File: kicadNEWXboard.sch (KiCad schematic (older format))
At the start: 24 parts, among them SW1 SW_Push, U1 ATmega32U4-AU, Y1 16MHz

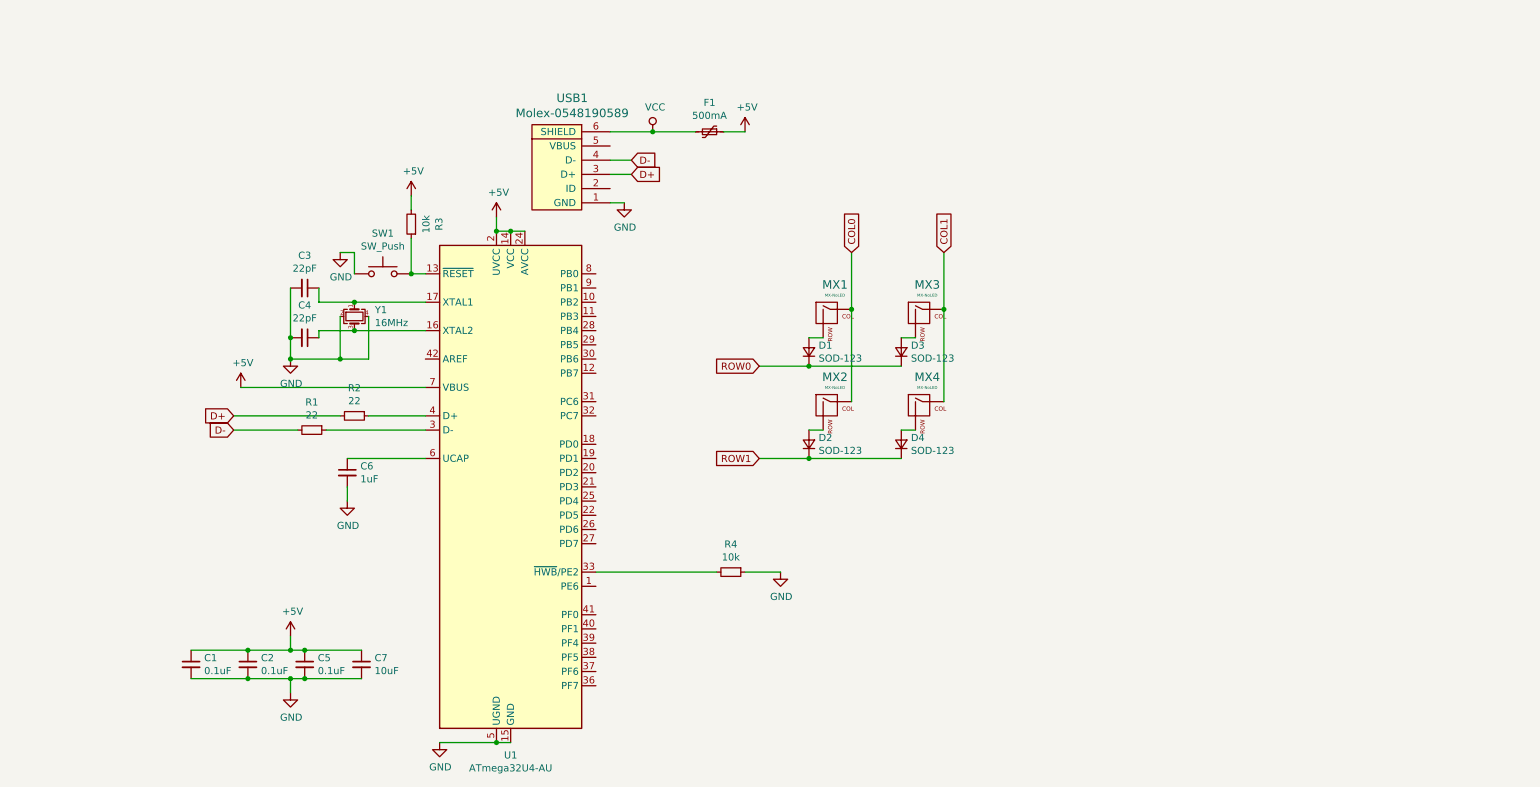
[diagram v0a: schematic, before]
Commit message: SVG
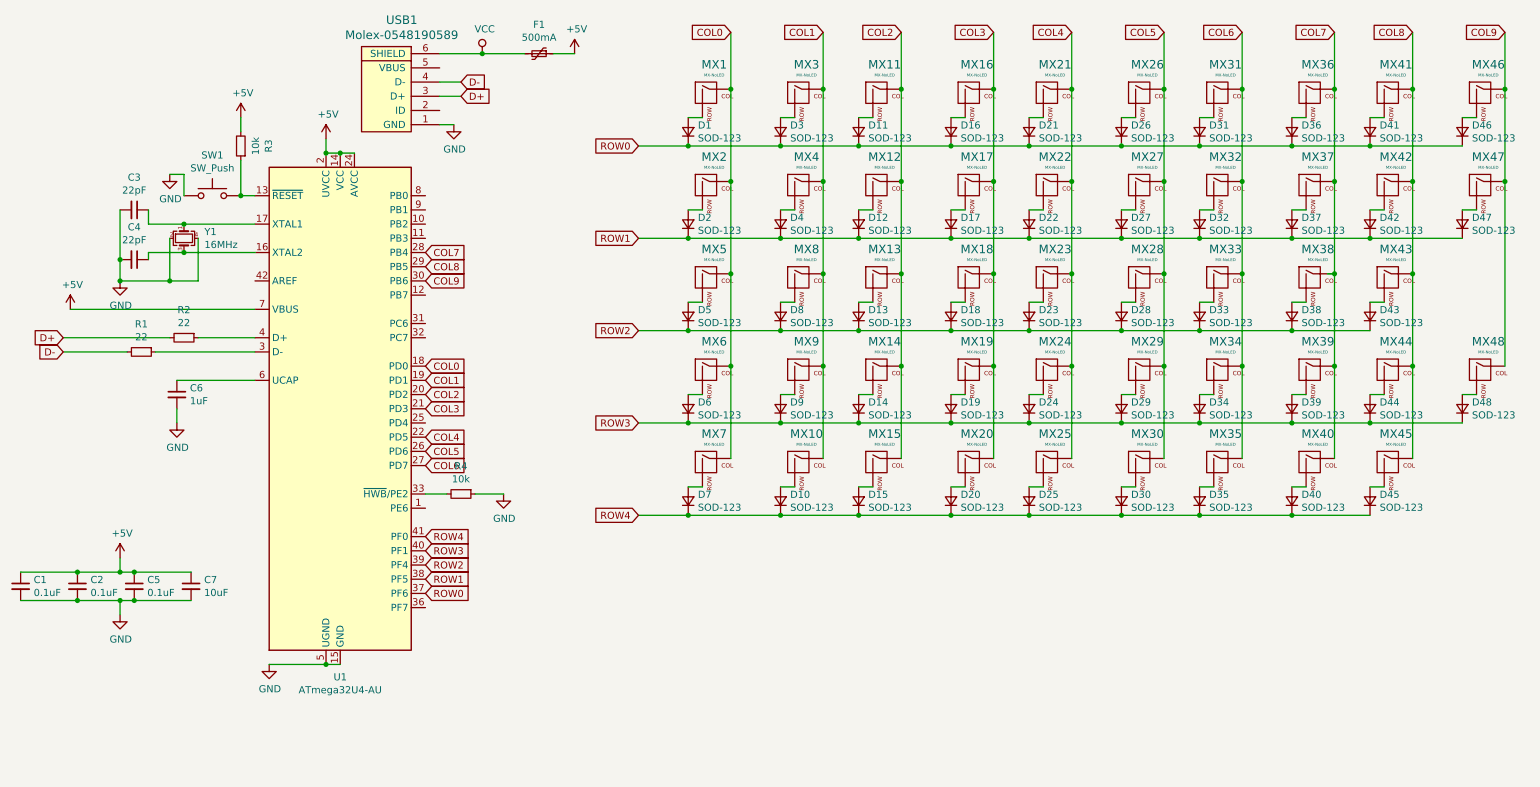
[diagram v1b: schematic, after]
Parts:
- added D10, D11, D12, D13, D14, D15, D16, D17, D18, D19, D20, D21, D22, D23, D24, D25, D26, D27, D28, D29, D30, D31, D32, D33, D34, D35, D36, D37, D38, D39, D40, D41, D42, D43, D44, D45, D46, D47, D48, D5, D6, D7, D8, D9: SOD-123, Diode_SMD:D_SOD-123, symbol Device:D_Small
- added MX10, MX11, MX12, MX13, MX14, MX15, MX16, MX17, MX18, MX19, MX20, MX21, MX22, MX23, MX24, MX25, MX26, MX27, MX28, MX29, MX30, MX31, MX32, MX33, MX34, MX35, MX36, MX37, MX38, MX39, MX40, MX41, MX42, MX43, MX44, MX45, MX46, MX47, MX48, MX5, MX6, MX7, MX8, MX9: MX-NoLED, MX_Alps_Hybrid:MX-1U, symbol MX_Alps_Hybrid:MX-NoLED
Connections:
- net COL0: now also U1.18 (PD0), MX5.1 (COL), MX6.1 (COL), MX7.1 (COL)
- net COL1: now also U1.19 (PD1), MX10.1 (COL), MX8.1 (COL), MX9.1 (COL)
- net ROW0: now also U1.37 (PF6), D11.1 (K), D16.1 (K), D21.1 (K), D26.1 (K), D31.1 (K), D36.1 (K), D41.1 (K), D46.1 (K)
- net ROW1: now also U1.38 (PF5), D12.1 (K), D17.1 (K), D22.1 (K), D27.1 (K), D32.1 (K), D37.1 (K), D42.1 (K), D47.1 (K)
- net COL2: now reaches U1.20 (PD2)
- net COL2: now also MX11.1 (COL), MX12.1 (COL), MX13.1 (COL), MX14.1 (COL), MX15.1 (COL)
- net COL3: now reaches U1.21 (PD3)
- net COL3: now also MX16.1 (COL), MX17.1 (COL), MX18.1 (COL), MX19.1 (COL), MX20.1 (COL)
- net COL4: now reaches U1.22 (PD5)
- net COL4: now also MX21.1 (COL), MX22.1 (COL), MX23.1 (COL), MX24.1 (COL), MX25.1 (COL)
- net COL5: now reaches U1.26 (PD6)
- net COL5: now also MX26.1 (COL), MX27.1 (COL), MX28.1 (COL), MX29.1 (COL), MX30.1 (COL)
- net COL6: now reaches U1.27 (PD7)
- net COL6: now also MX31.1 (COL), MX32.1 (COL), MX33.1 (COL), MX34.1 (COL), MX35.1 (COL)
- net COL7: now reaches U1.28 (PB4)
- net COL7: now also MX36.1 (COL), MX37.1 (COL), MX38.1 (COL), MX39.1 (COL), MX40.1 (COL)
- net COL8: now reaches U1.29 (PB5)
- net COL8: now also MX41.1 (COL), MX42.1 (COL), MX43.1 (COL), MX44.1 (COL), MX45.1 (COL)
- net COL9: now reaches U1.30 (PB6)
- net COL9: now also MX46.1 (COL), MX47.1 (COL), MX48.1 (COL)
- net ROW2: now reaches U1.39 (PF4)
- net ROW2: now also D13.1 (K), D18.1 (K), D23.1 (K), D28.1 (K), D33.1 (K), D38.1 (K), D43.1 (K), D5.1 (K), D8.1 (K)
- net ROW3: now reaches U1.40 (PF1)
- net ROW3: now also D14.1 (K), D19.1 (K), D24.1 (K), D29.1 (K), D34.1 (K), D39.1 (K), D44.1 (K), D48.1 (K), D6.1 (K), D9.1 (K)
- net ROW4: now reaches U1.41 (PF0)
- net ROW4: now also D10.1 (K), D15.1 (K), D20.1 (K), D25.1 (K), D30.1 (K), D35.1 (K), D40.1 (K), D45.1 (K), D7.1 (K)
- new net: D17.2 (A), MX17.2 (ROW)
- new net: D12.2 (A), MX12.2 (ROW)
- new net: D16.2 (A), MX16.2 (ROW)
- new net: D11.2 (A), MX11.2 (ROW)
- new net: D27.2 (A), MX27.2 (ROW)
- new net: D22.2 (A), MX22.2 (ROW)
- new net: D26.2 (A), MX26.2 (ROW)
- new net: D21.2 (A), MX21.2 (ROW)
- new net: D37.2 (A), MX37.2 (ROW)
- new net: D32.2 (A), MX32.2 (ROW)
- new net: D36.2 (A), MX36.2 (ROW)
- new net: D31.2 (A), MX31.2 (ROW)
- new net: D47.2 (A), MX47.2 (ROW)
- new net: D42.2 (A), MX42.2 (ROW)
- new net: D46.2 (A), MX46.2 (ROW)
- new net: D41.2 (A), MX41.2 (ROW)
- new net: D9.2 (A), MX9.2 (ROW)
- new net: D6.2 (A), MX6.2 (ROW)
- new net: D8.2 (A), MX8.2 (ROW)
- new net: D5.2 (A), MX5.2 (ROW)
- new net: D19.2 (A), MX19.2 (ROW)
- new net: D14.2 (A), MX14.2 (ROW)
- new net: D18.2 (A), MX18.2 (ROW)
- new net: D13.2 (A), MX13.2 (ROW)
- new net: D29.2 (A), MX29.2 (ROW)
- new net: D24.2 (A), MX24.2 (ROW)
- new net: D28.2 (A), MX28.2 (ROW)
- new net: D23.2 (A), MX23.2 (ROW)
- new net: D39.2 (A), MX39.2 (ROW)
- new net: D34.2 (A), MX34.2 (ROW)
- new net: D38.2 (A), MX38.2 (ROW)
- new net: D33.2 (A), MX33.2 (ROW)
- new net: D48.2 (A), MX48.2 (ROW)
- new net: D44.2 (A), MX44.2 (ROW)
- new net: D43.2 (A), MX43.2 (ROW)
- new net: D10.2 (A), MX10.2 (ROW)
- new net: D7.2 (A), MX7.2 (ROW)
- new net: D20.2 (A), MX20.2 (ROW)
- new net: D15.2 (A), MX15.2 (ROW)
- new net: D30.2 (A), MX30.2 (ROW)
- new net: D25.2 (A), MX25.2 (ROW)
- new net: D40.2 (A), MX40.2 (ROW)
- new net: D35.2 (A), MX35.2 (ROW)
- new net: D45.2 (A), MX45.2 (ROW)
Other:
- moved on the sheet: C1, C2, C3, C4, C5, C6, C7, D1, D2, D3, D4, F1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
